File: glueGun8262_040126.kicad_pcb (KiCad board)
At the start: 2 copper layers, 56 parts, among them CN1 KF243-5.0-2P, CN2 KF243-5.0-2P, CN3 KF243-5.0-2P, CN4 KF243-5.0-2P, CN5 KF243-5.0-2P, CN6 KF243-5.0-2P, CN7 KF243-5.0-2P, CN9 KF243-5.0-4P, U1 DRV8262DDWR, U10 INA240A2DR, U11 INA240A2DR, U2 DRV8262DDWR, U3 ESP32-S3-DEVKITC-1-N8R2, U5 6N137, U6 INA240A2DR, U7 INA240A2DR, U8 K7805-1000R3_C2992391, U9 TLP281-4(GB-TP,J,F

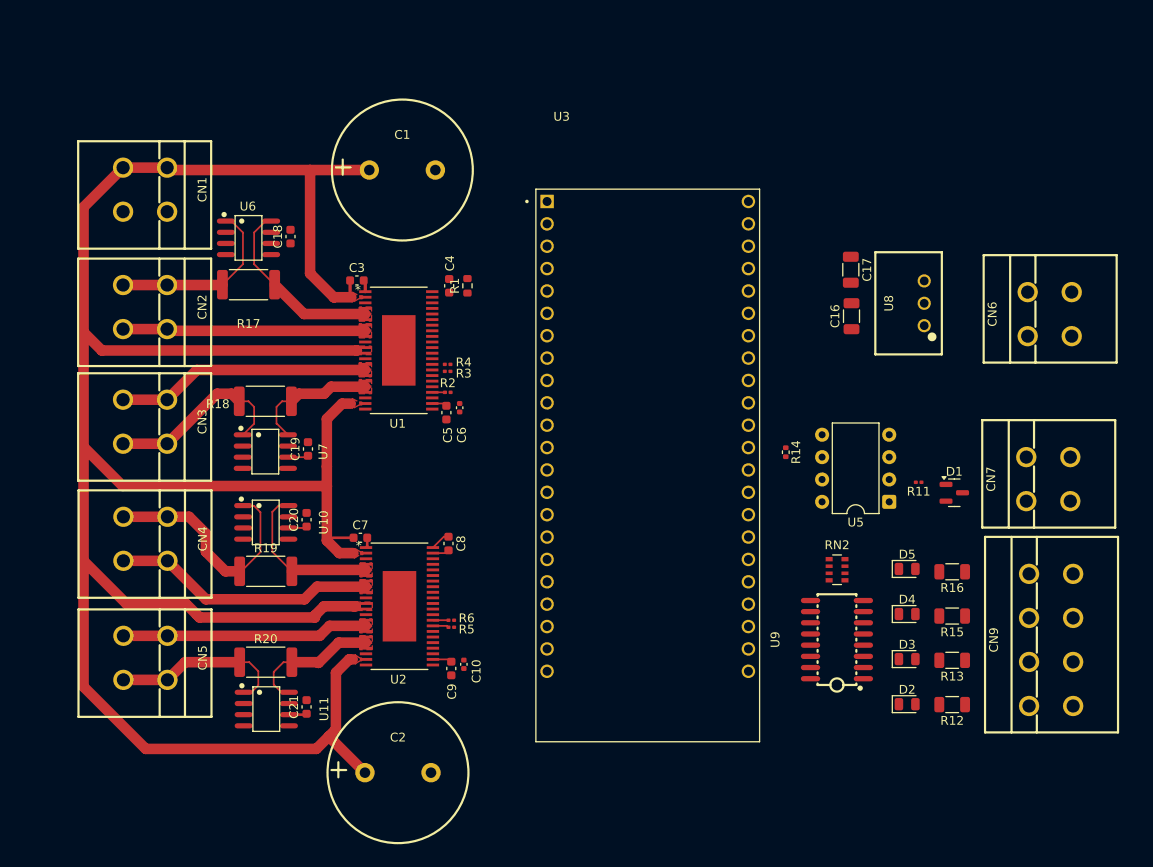
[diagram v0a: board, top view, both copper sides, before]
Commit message: cont rearrange pcb
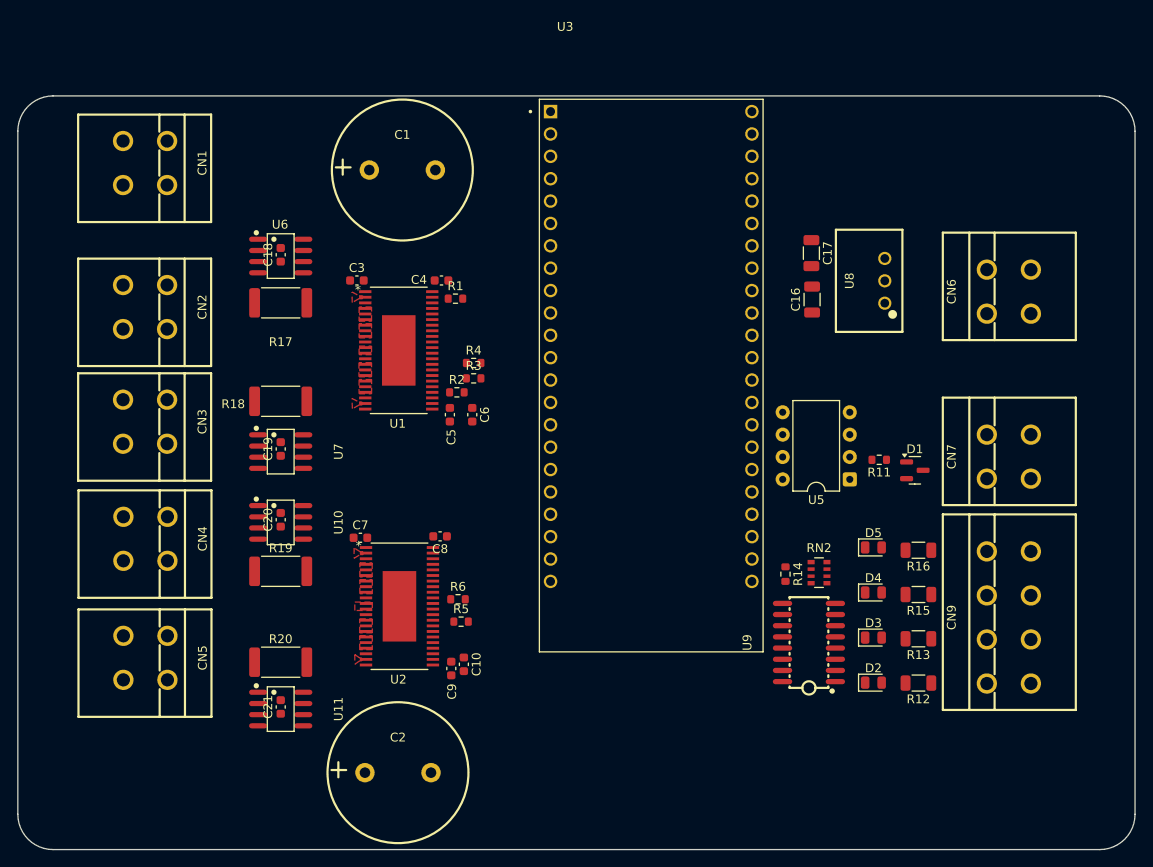
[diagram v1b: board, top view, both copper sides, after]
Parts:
- C10, C6: footprint Capacitor_SMD:C_0402_1005Metric -> Capacitor_SMD:C_0603_1608Metric
- R11, R2, R3, R4, R5, R6: footprint Resistor_SMD:R_0201_0603Metric -> Resistor_SMD:R_0603_1608Metric
- R14: footprint Resistor_SMD:R_0402_1005Metric -> Resistor_SMD:R_0603_1608Metric
- moved R14 13.8 mm to (193.4, 104.0)
- moved U3 10.2 mm to (178.1, 81.4)
- moved CN9 5.43 mm to (218.7, 108.9)
- moved CN6 5.29 mm to (218.7, 71.9)
- moved D1 5.15 mm to (208.0, 92.2)
- moved U5 5.15 mm to (200.7, 93.2)
- moved R11 5.15 mm to (204.0, 91.0)
- moved U8 5.15 mm to (204.6, 70.7)
- moved CN7 5.15 mm to (218.7, 90.6)
- moved C16 4.86 mm to (196.4, 72.8)
- moved C17 4.86 mm to (196.3, 67.5)
- moved D2 4.55 mm to (203.3, 116.3)
- moved D4 4.55 mm to (203.3, 106.1)
- moved R16 4.55 mm to (208.5, 101.3)
- moved D3 4.55 mm to (203.3, 111.2)
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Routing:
- net +48V: track 275.5 -> 0.00 mm
- net /U2_OUT2: track 29.9 -> 0.00 mm
- net /U1_OUT4: track 28.9 -> 0.00 mm
- net /U2_OUT4: track 28.0 -> 0.00 mm
- net /U1_OUT2: track 28.0 -> 0.00 mm
- net Net-(U10-IN-): track 26.4 -> 0.00 mm
- net Net-(U7-IN-): track 21.6 -> 0.00 mm
- net Net-(U6-IN-): track 21.4 -> 0.00 mm
- net /U1_OUT1: track 21.0 -> 0.00 mm
- net Net-(U11-IN-): track 20.2 -> 0.00 mm
- net /U2_OUT1: track 18.3 -> 0.00 mm
- net /U2_OUT3: track 15.4 -> 0.00 mm
- net /U1_OUT3: track 14.8 -> 0.00 mm
- net +3V3: track 6.51 -> 0.00 mm
- net Net-(U2-CPH/GND): track 2.27 -> 0.00 mm
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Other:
- board outline added: 126.8 x 85.6 mm

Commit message: cont
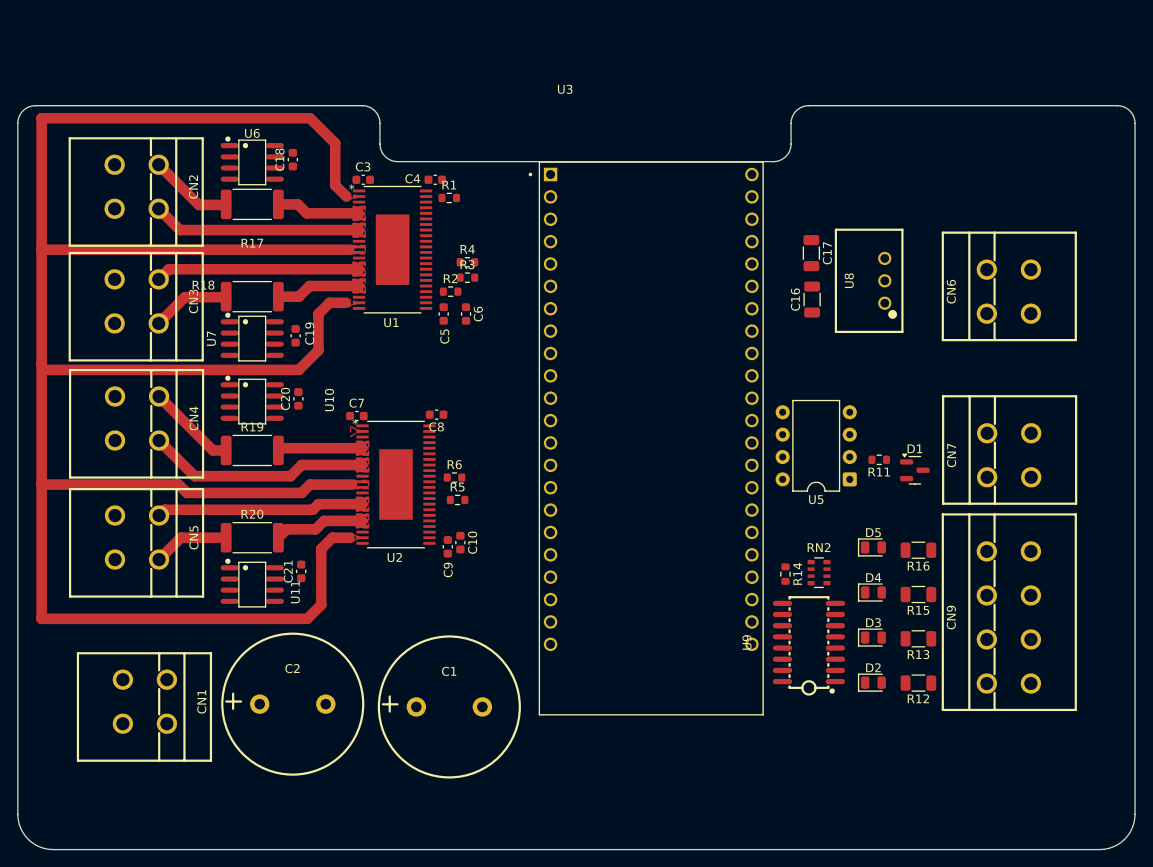
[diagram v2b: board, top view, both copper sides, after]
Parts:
- moved C1 61.2 mm to (155.2, 119.1)
- moved CN1 61.2 mm to (120.6, 118.5)
- moved C21 15.6 mm to (138.4, 103.7)
- moved U11 14.5 mm to (132.8, 105.2)
- moved R20 14.5 mm to (132.8, 99.8)
- moved C2 14.3 mm to (137.4, 118.7)
- moved U10 14.1 mm to (132.8, 84.4)
- moved R19 14.1 mm to (132.8, 89.9)
- moved C20 13.9 mm to (138.1, 84.1)
- moved C10 13.8 mm to (156.4, 100.4)
- moved C7 13.8 mm to (144.7, 86.0)
- moved C9 13.8 mm to (155.0, 100.9)
- moved R5 13.8 mm to (156.1, 95.6)
- moved R6 13.8 mm to (155.8, 93.0)
- moved C8 13.8 mm to (153.7, 85.9)
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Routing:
- net +48V: track 0.00 -> 250.8 mm
- net /U2_OUT2: track 0.00 -> 25.3 mm
- net /U1_OUT2: track 0.00 -> 23.8 mm
- net /U2_OUT4: track 0.00 -> 23.6 mm
- net /U1_OUT4: track 0.00 -> 23.2 mm
- net /U2_OUT3: track 0.00 -> 10.3 mm
- net Net-(U10-IN-): track 0.00 -> 10.2 mm
- net /U1_OUT3: track 0.00 -> 9.67 mm
- net /U2_OUT1: track 0.00 -> 9.66 mm
- net /U1_OUT1: track 0.00 -> 9.59 mm
- net Net-(U6-IN-): track 0.00 -> 9.58 mm
- net Net-(U7-IN-): track 0.00 -> 8.92 mm
- net Net-(U11-IN-): track 0.00 -> 8.65 mm
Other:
- board size 126.8 x 85.6 mm -> 126.8 x 84.5 mm
